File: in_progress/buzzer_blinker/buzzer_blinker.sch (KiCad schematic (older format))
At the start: 12 parts, among them SW1 SW_PUSH, SW2 SWITCH_INV

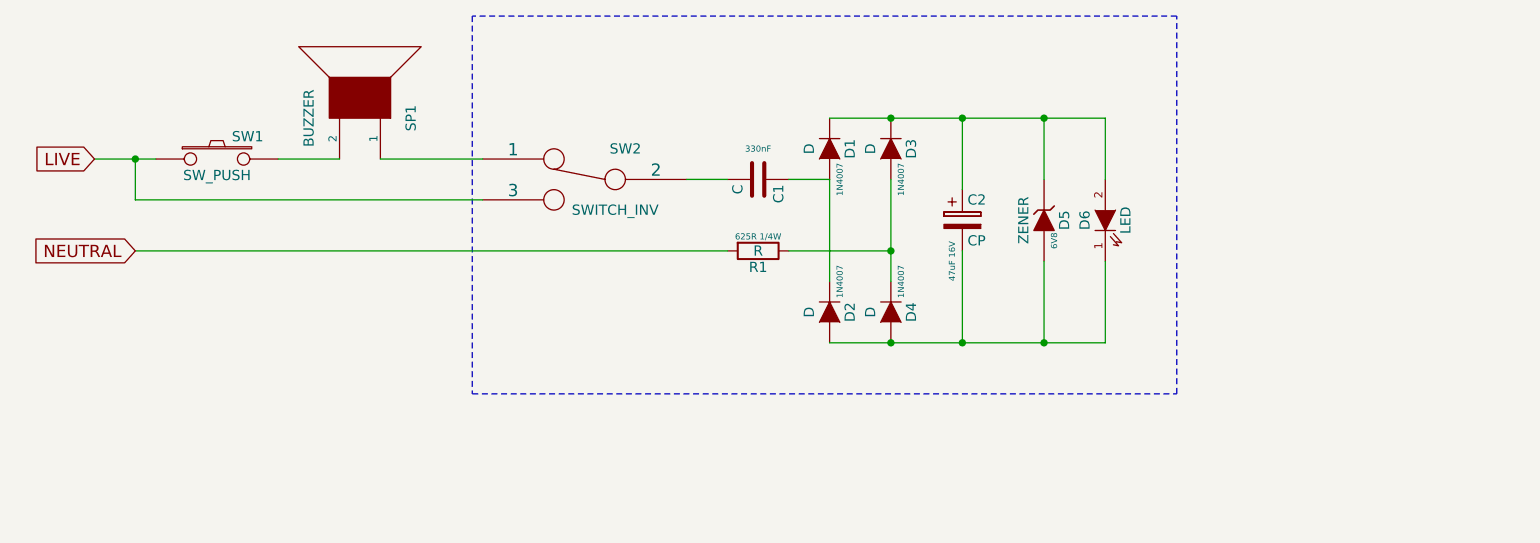
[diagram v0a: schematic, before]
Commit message: .
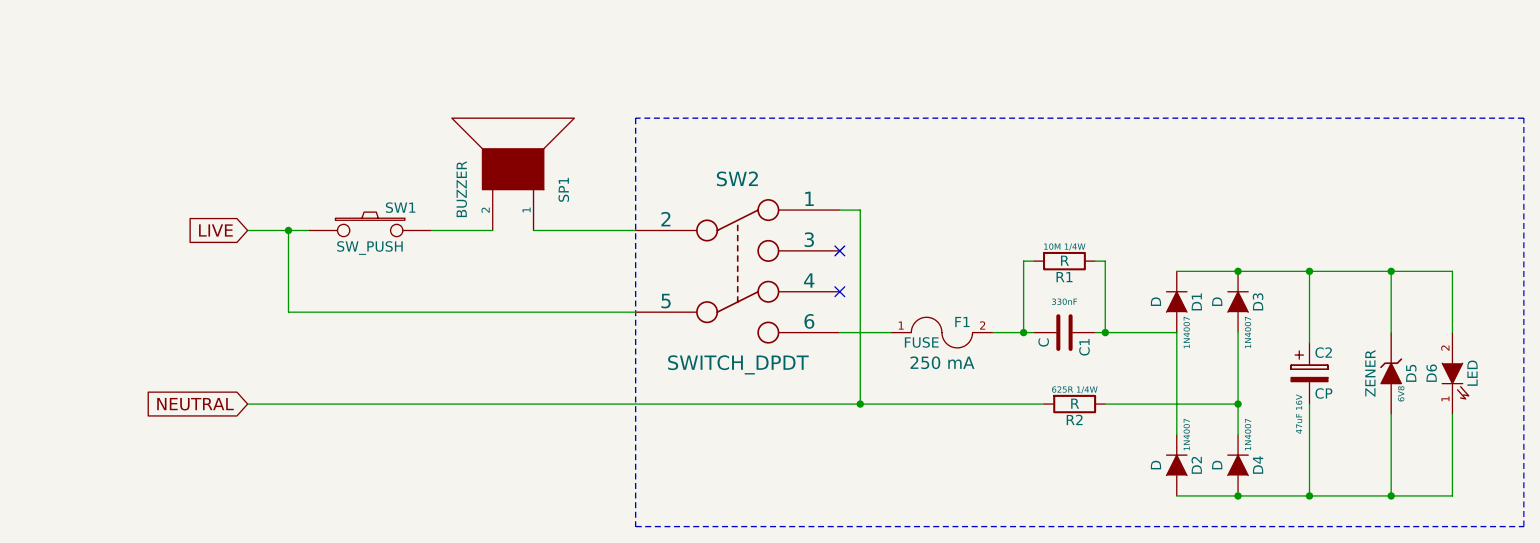
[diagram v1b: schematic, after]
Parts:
- removed SW2: SWITCH_INV, symbol SWITCH_INV
- added F1: FUSE, 250 mA, symbol FUSE
- added R1: R, 10M 1/4W, symbol R
- added SW2: SWITCH_DPDT, symbol SWITCH_DPDT
- renumbered R1 to R2
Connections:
- net LIVE: now also SW2.5
- net NEUTRAL: now also SW2.1
- net at C1.1, D1.2 (A), D2.1 (K): now also R1.1
- net at C1.2: now also F1.2, R1.2
- net at SP1.1: now also SW2.2
- new net: F1.1, SW2.6
- no-connect marks 0 -> 2
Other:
- moved on the sheet: C1, C2, D1, D2, D3, D4, D5, D6, R2, SP1, SW1
